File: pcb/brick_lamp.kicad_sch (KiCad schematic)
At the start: 11 parts, among them J1 LED_24V_OUT, J2 24V_IN, J3 DEBUG, J4 DEBUG, Q1 CSD17302Q5A, U2 MCP1799x-330xxTT, U3 ATtiny85V-10S

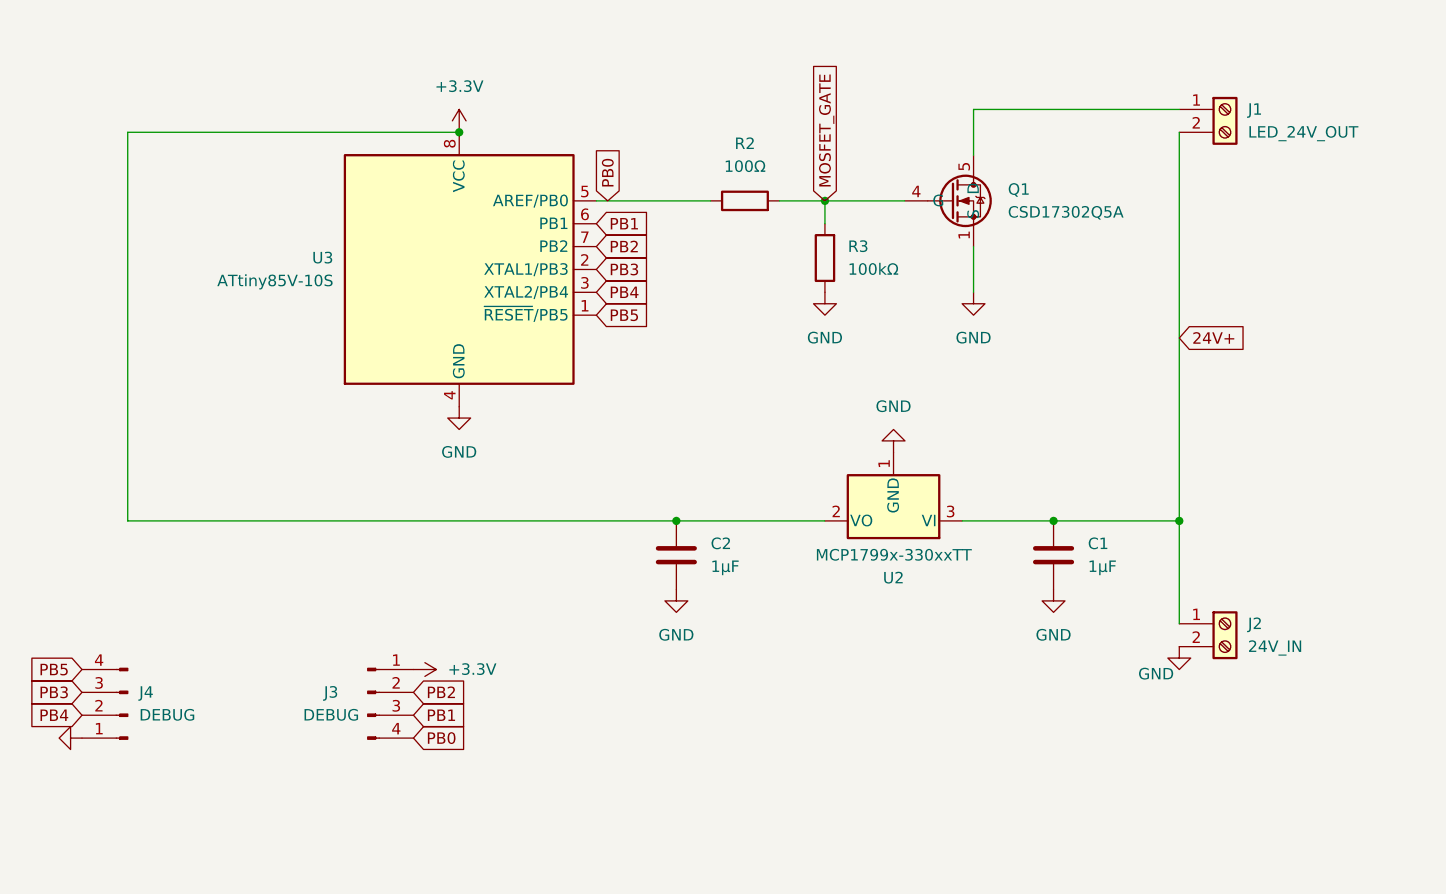
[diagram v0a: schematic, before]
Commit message: Cleanup schematics
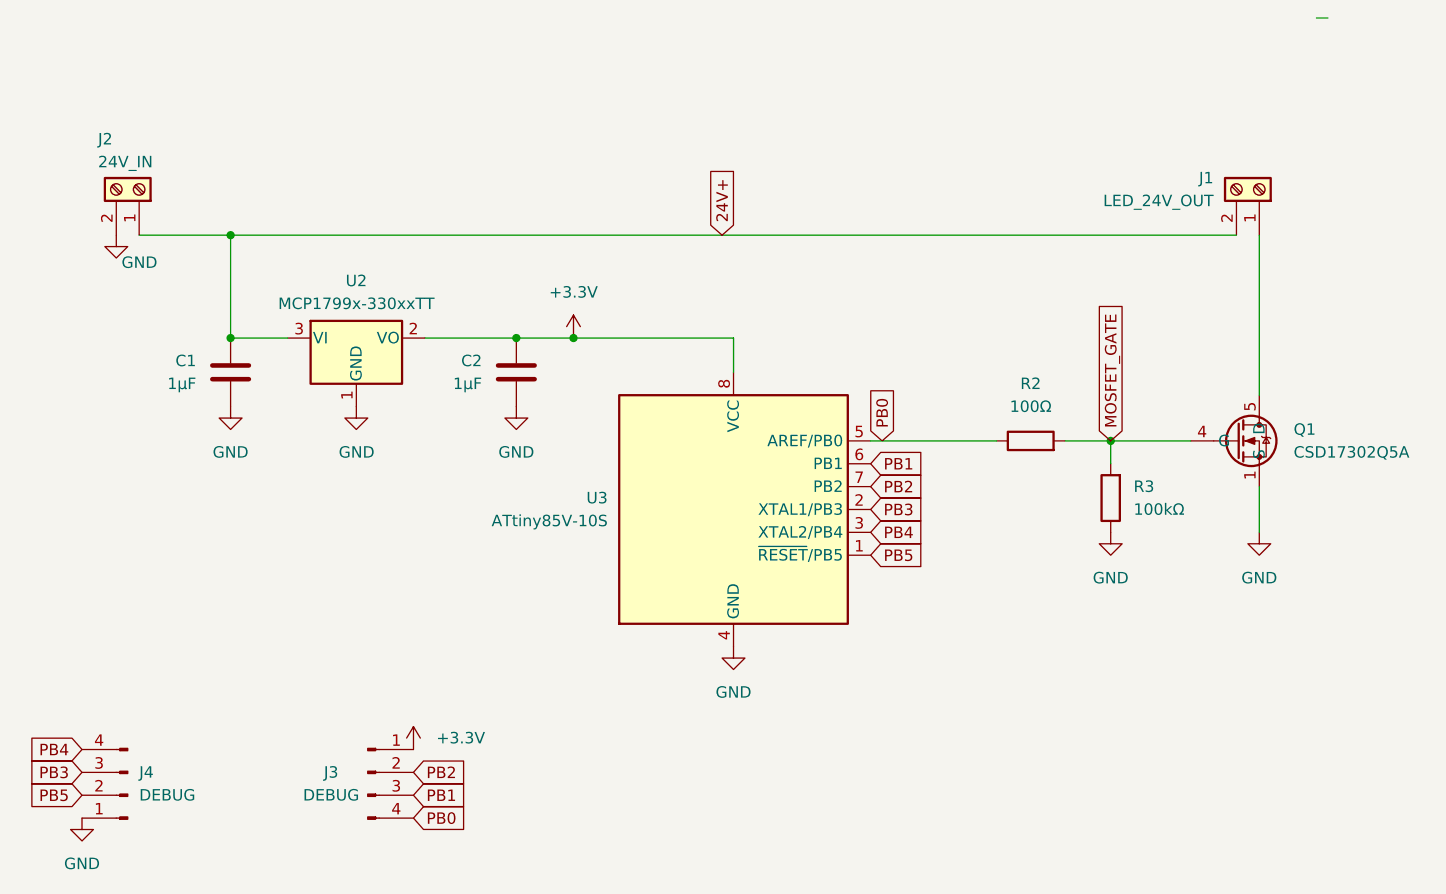
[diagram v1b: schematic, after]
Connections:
- net PB4: now also J4.4 (Pin_4); no longer J4.2 (Pin_2)
- net PB5: now also J4.2 (Pin_2); no longer J4.4 (Pin_4)
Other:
- moved on the sheet: C1, C2, J1, J2, J3, J4, Q1, R2, R3, U2, U3
